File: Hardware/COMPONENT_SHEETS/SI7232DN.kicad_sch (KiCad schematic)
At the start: 9 parts, among them Q1 SI7232DN-T1-GE3

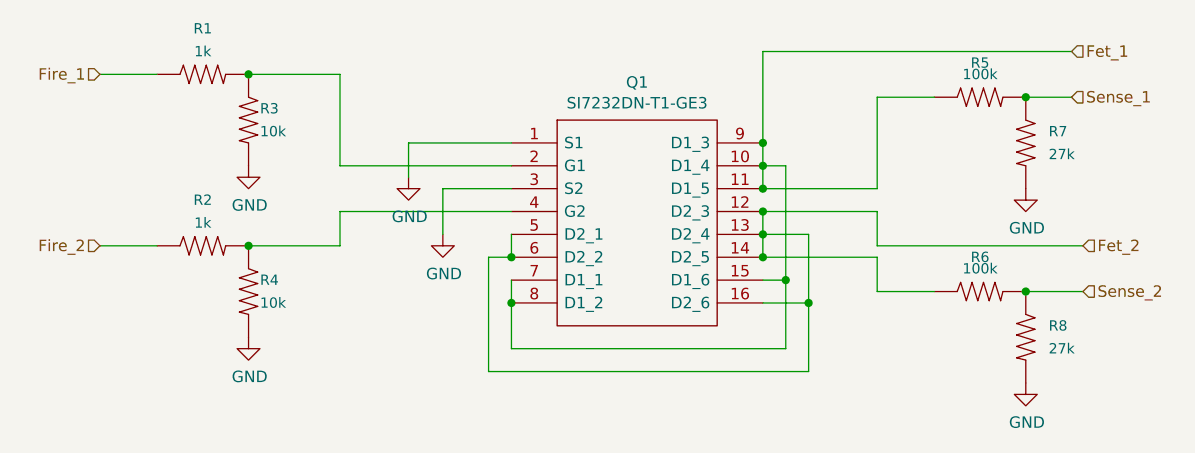
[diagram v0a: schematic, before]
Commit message: Adjusted silkscreen labels, corrected MCU pinout, added pull up resistor to bootloader line, added usb cut out
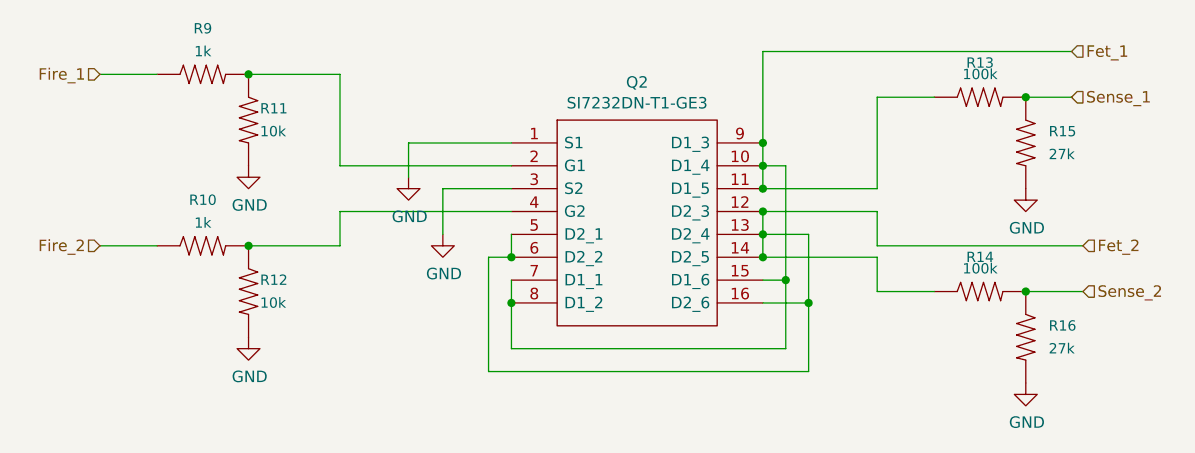
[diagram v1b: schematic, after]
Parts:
- renumbered Q1 to Q2, R2 to R10, R3 to R11, R4 to R12, R5 to R13, R6 to R14, R7 to R15, R8 to R16, R1 to R9
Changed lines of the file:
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@@
   (symbol (lib_id "Charges_KiCAD_Project-rescue:RESISTOR0402-SparkFun-Resistors") (at 113.03 78.74 270)
     (in_bom yes) (on_board yes)
-    (property "Reference" "R3" (id 0) (at 114.3 77.47 90)
+    (property "Reference" "R11" (id 0) (at 114.3 77.47 90)
       (effects (font (size 1.143 1.143)) (justify left))
     )
@@
   (symbol (lib_id "Charges_KiCAD_Project-rescue:RESISTOR0402-SparkFun-Resistors") (at 107.95 73.66 0)
     (in_bom yes) (on_board yes)
-    (property "Reference" "R1" (id 0) (at 107.95 68.58 0)
+    (property "Reference" "R9" (id 0) (at 107.95 68.58 0)
       (effects (font (size 1.143 1.143)))
     )
@@
   (symbol (lib_id "Charges_KiCAD_Project-rescue:RESISTOR0402-SparkFun-Resistors") (at 113.03 97.79 270)
     (in_bom yes) (on_board yes)
-    (property "Reference" "R4" (id 0) (at 114.3 96.52 90)
+    (property "Reference" "R12" (id 0) (at 114.3 96.52 90)
       (effects (font (size 1.143 1.143)) (justify left))
     )
@@
   (symbol (lib_id "Charges_KiCAD_Project-rescue:SI7232DN-T1-GE3-SamacSys_Parts") (at 142.24 81.28 0)
     (in_bom yes) (on_board yes)
-    (property "Reference" "Q1" (id 0) (at 156.21 74.549 0))
+    (property "Reference" "Q2" (id 0) (at 156.21 74.549 0))
     (property "Value" "SI7232DN-T1-GE3" (id 1) (at 156.21 76.8604 0))
     (property "Footprint" "SamacSys_Parts:SI7232DNT1GE3" (id 2) (at 166.37 78.74 0)
@@
   (symbol (lib_id "Charges_KiCAD_Project-rescue:RESISTOR0402-SparkFun-Resistors") (at 199.39 102.87 270)
     (in_bom yes) (on_board yes)
-    (property "Reference" "R8" (id 0) (at 201.93 101.6 90)
+    (property "Reference" "R16" (id 0) (at 201.93 101.6 90)
       (effects (font (size 1.143 1.143)) (justify left))
     )
@@
   (symbol (lib_id "Charges_KiCAD_Project-rescue:RESISTOR0402-SparkFun-Resistors") (at 107.95 92.71 0)
     (in_bom yes) (on_board yes)
-    (property "Reference" "R2" (id 0) (at 107.95 87.63 0)
+    (property "Reference" "R10" (id 0) (at 107.95 87.63 0)
       (effects (font (size 1.143 1.143)))
     )
@@
   (symbol (lib_id "Charges_KiCAD_Project-rescue:RESISTOR0402-SparkFun-Resistors") (at 194.31 76.2 0)
     (in_bom yes) (on_board yes)
-    (property "Reference" "R5" (id 0) (at 194.31 72.39 0)
+    (property "Reference" "R13" (id 0) (at 194.31 72.39 0)
       (effects (font (size 1.143 1.143)))
     )
@@
   (symbol (lib_id "Charges_KiCAD_Project-rescue:RESISTOR0402-SparkFun-Resistors") (at 199.39 81.28 270)
     (in_bom yes) (on_board yes)
-    (property "Reference" "R7" (id 0) (at 201.93 80.01 90)
+    (property "Reference" "R15" (id 0) (at 201.93 80.01 90)
       (effects (font (size 1.143 1.143)) (justify left))
     )
@@
   (symbol (lib_id "Charges_KiCAD_Project-rescue:RESISTOR0402-SparkFun-Resistors") (at 194.31 97.79 0)
     (in_bom yes) (on_board yes)
-    (property "Reference" "R6" (id 0) (at 194.31 93.98 0)
-      (effects (font (size 1.143 1.143)))
-    )
+    (property "Reference" "R14" (id 0) (at 194.31 93.98 0)
+      (effects (font (size 1.143 1.143)))
+    )

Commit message: Added bleed off resistors to charge capacitors
R = -t/C*ln(V/Vo) = (-1)/(0.0015)*ln(1v/5v) = 1072.96 ≈ 1000 ohm
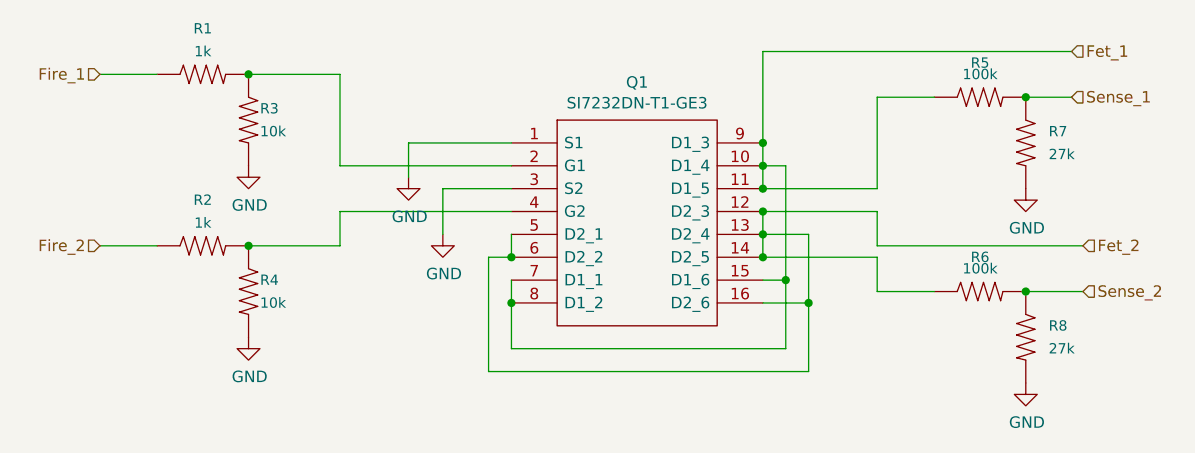
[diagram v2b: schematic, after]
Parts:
- renumbered Q2 to Q1, R9 to R1, R10 to R2, R11 to R3, R12 to R4, R13 to R5, R14 to R6, R15 to R7, R16 to R8
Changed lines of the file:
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@@
   (symbol (lib_id "Charges_KiCAD_Project-rescue:RESISTOR0402-SparkFun-Resistors") (at 113.03 78.74 270)
     (in_bom yes) (on_board yes)
-    (property "Reference" "R11" (id 0) (at 114.3 77.47 90)
+    (property "Reference" "R3" (id 0) (at 114.3 77.47 90)
       (effects (font (size 1.143 1.143)) (justify left))
     )
@@
   (symbol (lib_id "Charges_KiCAD_Project-rescue:RESISTOR0402-SparkFun-Resistors") (at 107.95 73.66 0)
     (in_bom yes) (on_board yes)
-    (property "Reference" "R9" (id 0) (at 107.95 68.58 0)
+    (property "Reference" "R1" (id 0) (at 107.95 68.58 0)
       (effects (font (size 1.143 1.143)))
     )
@@
   (symbol (lib_id "Charges_KiCAD_Project-rescue:RESISTOR0402-SparkFun-Resistors") (at 113.03 97.79 270)
     (in_bom yes) (on_board yes)
-    (property "Reference" "R12" (id 0) (at 114.3 96.52 90)
+    (property "Reference" "R4" (id 0) (at 114.3 96.52 90)
       (effects (font (size 1.143 1.143)) (justify left))
     )
@@
   (symbol (lib_id "Charges_KiCAD_Project-rescue:SI7232DN-T1-GE3-SamacSys_Parts") (at 142.24 81.28 0)
     (in_bom yes) (on_board yes)
-    (property "Reference" "Q2" (id 0) (at 156.21 74.549 0))
+    (property "Reference" "Q1" (id 0) (at 156.21 74.549 0))
     (property "Value" "SI7232DN-T1-GE3" (id 1) (at 156.21 76.8604 0))
     (property "Footprint" "SamacSys_Parts:SI7232DNT1GE3" (id 2) (at 166.37 78.74 0)
@@
   (symbol (lib_id "Charges_KiCAD_Project-rescue:RESISTOR0402-SparkFun-Resistors") (at 199.39 102.87 270)
     (in_bom yes) (on_board yes)
-    (property "Reference" "R16" (id 0) (at 201.93 101.6 90)
+    (property "Reference" "R8" (id 0) (at 201.93 101.6 90)
       (effects (font (size 1.143 1.143)) (justify left))
     )
@@
   (symbol (lib_id "Charges_KiCAD_Project-rescue:RESISTOR0402-SparkFun-Resistors") (at 107.95 92.71 0)
     (in_bom yes) (on_board yes)
-    (property "Reference" "R10" (id 0) (at 107.95 87.63 0)
+    (property "Reference" "R2" (id 0) (at 107.95 87.63 0)
       (effects (font (size 1.143 1.143)))
     )
@@
   (symbol (lib_id "Charges_KiCAD_Project-rescue:RESISTOR0402-SparkFun-Resistors") (at 194.31 76.2 0)
     (in_bom yes) (on_board yes)
-    (property "Reference" "R13" (id 0) (at 194.31 72.39 0)
+    (property "Reference" "R5" (id 0) (at 194.31 72.39 0)
       (effects (font (size 1.143 1.143)))
     )
@@
   (symbol (lib_id "Charges_KiCAD_Project-rescue:RESISTOR0402-SparkFun-Resistors") (at 199.39 81.28 270)
     (in_bom yes) (on_board yes)
-    (property "Reference" "R15" (id 0) (at 201.93 80.01 90)
+    (property "Reference" "R7" (id 0) (at 201.93 80.01 90)
       (effects (font (size 1.143 1.143)) (justify left))
     )
@@
   (symbol (lib_id "Charges_KiCAD_Project-rescue:RESISTOR0402-SparkFun-Resistors") (at 194.31 97.79 0)
     (in_bom yes) (on_board yes)
-    (property "Reference" "R14" (id 0) (at 194.31 93.98 0)
-      (effects (font (size 1.143 1.143)))
-    )
+    (property "Reference" "R6" (id 0) (at 194.31 93.98 0)
+      (effects (font (size 1.143 1.143)))
+    )
